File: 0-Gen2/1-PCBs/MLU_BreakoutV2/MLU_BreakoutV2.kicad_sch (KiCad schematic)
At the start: 17 parts, among them J13 SBH11-PBPC-D10-ST-BK, J7 SBH11-PBPC-D10-ST-BK, U6 Teensy4.1

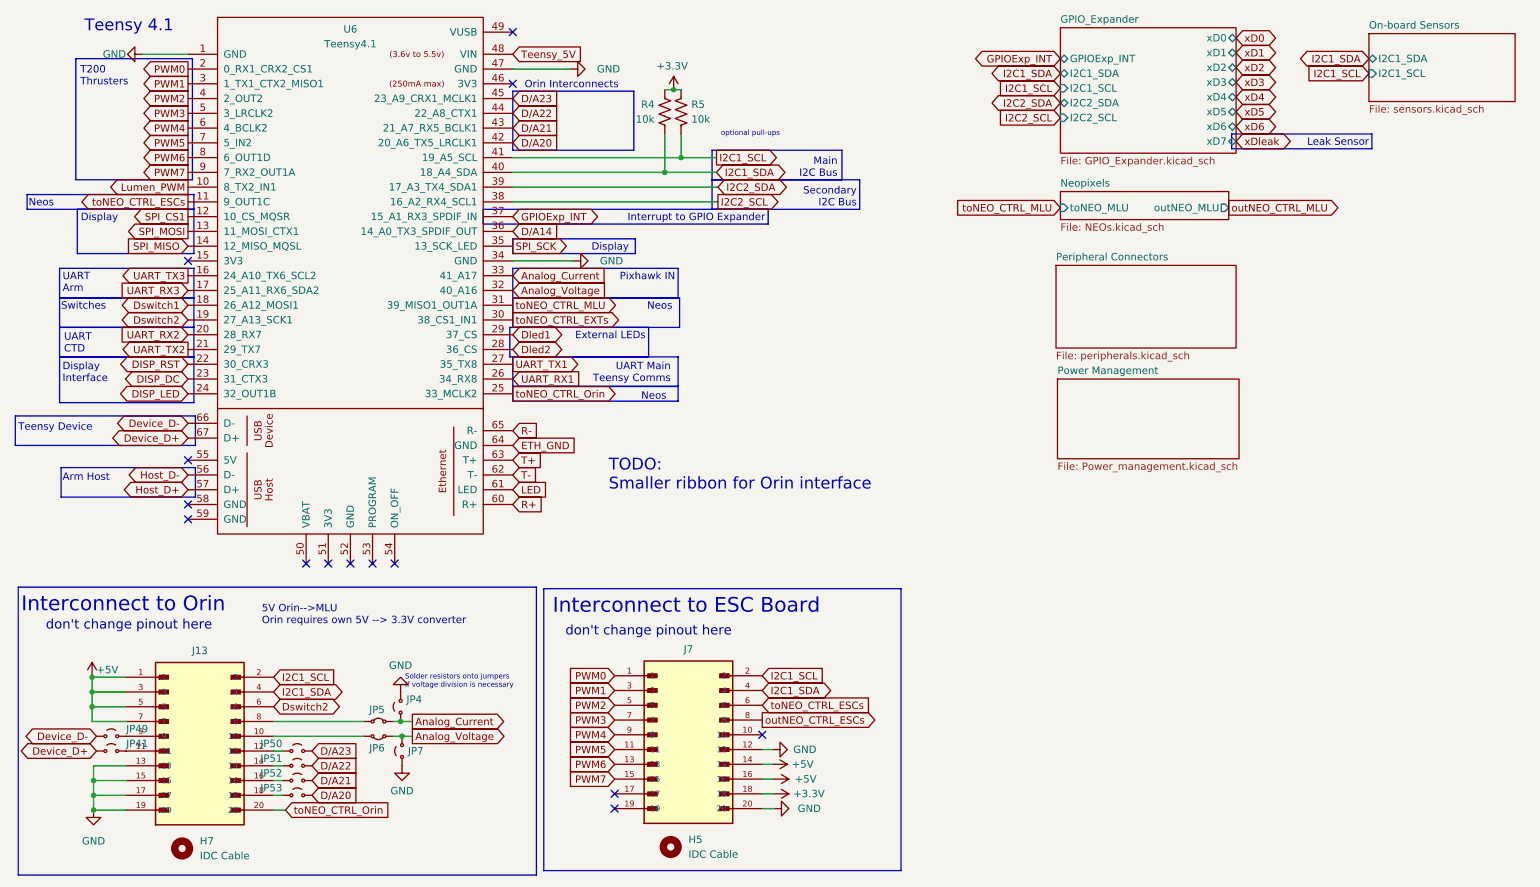
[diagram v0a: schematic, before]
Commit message: before restructure
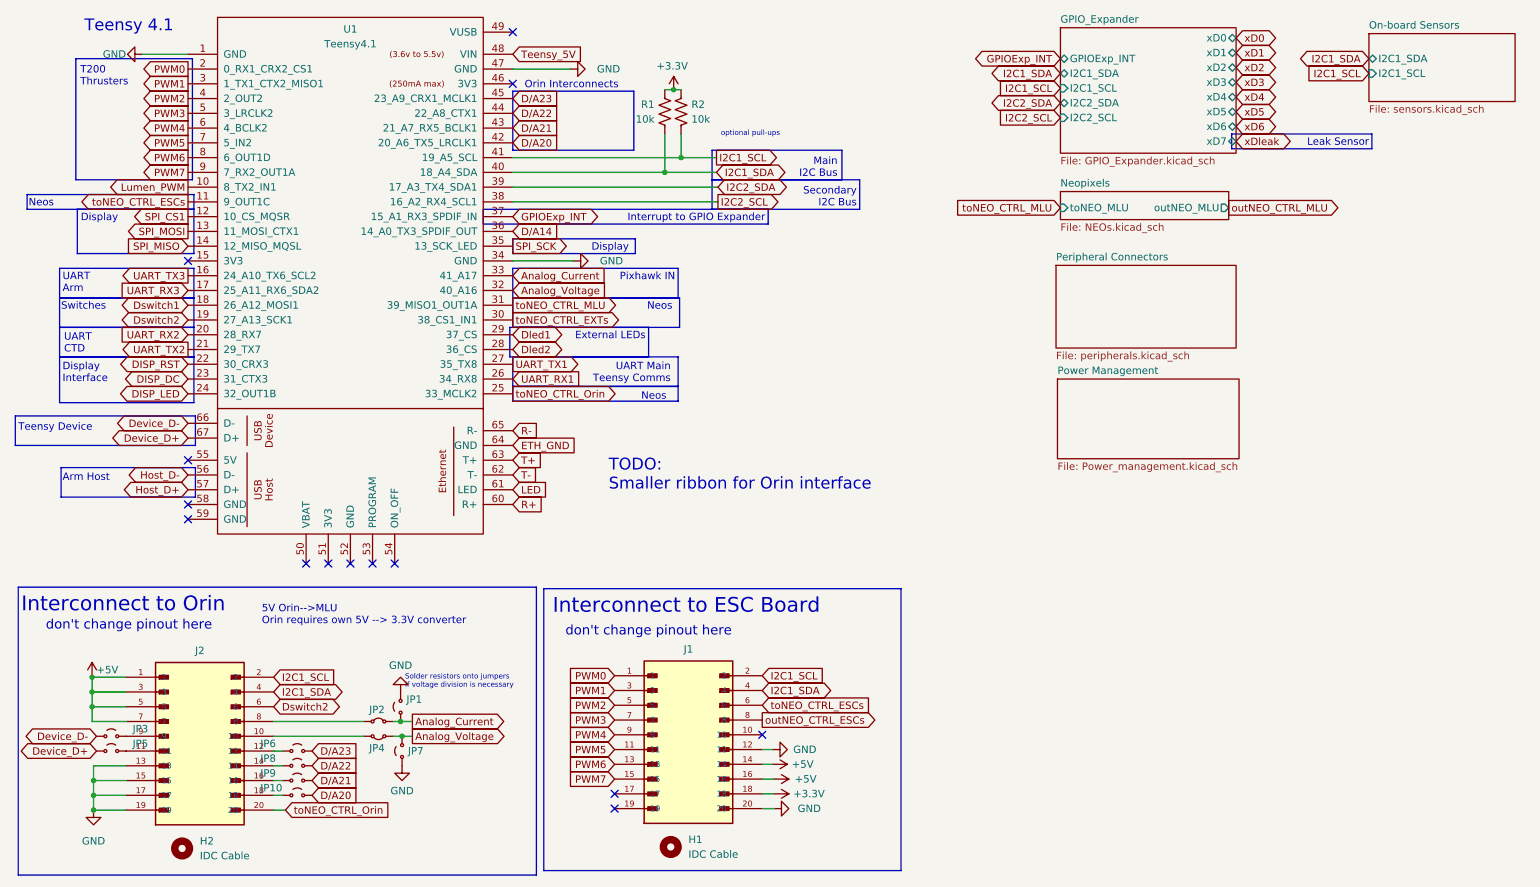
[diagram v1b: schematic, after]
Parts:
- renumbered H5 to H1, H7 to H2, J7 to J1, J13 to J2, JP4 to JP1, JP53 to JP10, JP5 to JP2, JP49 to JP3, JP6 to JP4, JP41 to JP5, JP50 to JP6, JP51 to JP8, JP52 to JP9, R4 to R1, R5 to R2, U6 to U1
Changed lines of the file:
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@@
 		(dnp no)
 		(fields_autoplaced yes)
-		(property "Reference" "#PWR039"
+		(property "Reference" "#PWR04"
 			(at 116.84 56.388 0)
 			(effects
@@
 			(project "MLU_BreakoutV2"
 				(path "/55121ba7-5d22-4fe3-93aa-7f76d75b410c"
-					(reference "#PWR039")
+					(reference "#PWR04")
 					(unit 1)
 				)
@@
 		(on_board yes)
 		(dnp no)
-		(property "Reference" "U6"
+		(property "Reference" "U1"
 			(at 72.136 16.51 0)
 			(effects
@@
 			(project "MLU_BreakoutV2"
 				(path "/55121ba7-5d22-4fe3-93aa-7f76d75b410c"
-					(reference "U6")
+					(reference "U1")
 					(unit 1)
 				)
@@
 		(on_board yes)
 		(dnp no)
-		(property "Reference" "#PWR027"
+		(property "Reference" "#PWR03"
 			(at 127.762 30.988 0)
 			(effects
@@
 			(project "MLU_BreakoutV2"
 				(path "/55121ba7-5d22-4fe3-93aa-7f76d75b410c"
-					(reference "#PWR027")
+					(reference "#PWR03")
 					(unit 1)
 				)
@@
 		(on_board yes)
 		(dnp no)
-		(property "Reference" "R4"
+		(property "Reference" "R1"
 			(at 124.46 29.4639 0)
 			(effects
@@
 			(project "MLU_BreakoutV2"
 				(path "/55121ba7-5d22-4fe3-93aa-7f76d75b410c"
-					(reference "R4")
+					(reference "R1")
 					(unit 1)
 				)
@@
 		(dnp no)
 		(fields_autoplaced yes)
-		(property "Reference" "H7"
+		(property "Reference" "H2"
 			(at 46.228 156.2099 0)
 			(effects
@@
 			(project "MLU_BreakoutV2"
 				(path "/55121ba7-5d22-4fe3-93aa-7f76d75b410c"
-					(reference "H7")
+					(reference "H2")
 					(unit 1)
 				)
@@
 		(dnp no)
 		(fields_autoplaced yes)
-		(property "Reference" "#PWR063"
+		(property "Reference" "#PWR09"
 			(at 81.026 149.606 0)
 			(effects
@@
 			(project ""
 				(path "/55121ba7-5d22-4fe3-93aa-7f76d75b410c"
-					(reference "#PWR063")
+					(reference "#PWR09")
 					(unit 1)
 				)
@@
 		(dnp no)
 		(fields_autoplaced yes)
-		(property "Reference" "#PWR061"
+		(property "Reference" "#PWR06"
 			(at 80.772 124.206 0)
 			(effects
@@
 			(project ""
 				(path "/55121ba7-5d22-4fe3-93aa-7f76d75b410c"
-					(reference "#PWR061")
+					(reference "#PWR06")
 					(unit 1)
 				)
@@
 		(dnp no)
 		(fields_autoplaced yes)
-		(property "Reference" "#PWR030"
+		(property "Reference" "#PWR010"
 			(at 141.224 145.542 0)
 			(effects
@@
 			(project "MLU_BreakoutV2"
 				(path "/55121ba7-5d22-4fe3-93aa-7f76d75b410c"
-					(reference "#PWR030")
+					(reference "#PWR010")
 					(unit 1)
 				)
@@
 		(on_board yes)
 		(dnp no)
-		(property "Reference" "JP5"
+		(property "Reference" "JP2"
 			(at 76.708 133.604 0)
 			(effects
@@
 			(project ""
 				(path "/55121ba7-5d22-4fe3-93aa-7f76d75b410c"
-					(reference "JP5")
+					(reference "JP2")
 					(unit 1)
 				)
@@
 		(on_board yes)
 		(dnp no)
-		(property "Reference" "#PWR060"
+		(property "Reference" "#PWR05"
 			(at 27.686 131.826 0)
 			(effects
@@
 			(project "MLU_BreakoutV2"
 				(path "/55121ba7-5d22-4fe3-93aa-7f76d75b410c"
-					(reference "#PWR060")
+					(reference "#PWR05")
 					(unit 1)
 				)
@@
 		(on_board yes)
 		(dnp no)
-		(property "Reference" "JP50"
+		(property "Reference" "JP6"
 			(at 56.642 139.446 0)
 			(effects
@@
 			(project "MLU_BreakoutV2"
 				(path "/55121ba7-5d22-4fe3-93aa-7f76d75b410c"
-					(reference "JP50")
+					(reference "JP6")
 					(unit 1)
 				)
@@
 		(dnp no)
 		(fields_autoplaced yes)
-		(property "Reference" "#PWR028"
+		(property "Reference" "#PWR07"
 			(at 151.13 140.462 0)
 			(effects
@@
 			(project "MLU_BreakoutV2"
 				(path "/55121ba7-5d22-4fe3-93aa-7f76d75b410c"
-					(reference "#PWR028")
+					(reference "#PWR07")
 					(unit 1)
 				)
@@
 		(on_board yes)
 		(dnp no)
-		(property "Reference" "JP4"
+		(property "Reference" "JP1"
 			(at 81.788 131.826 90)
 			(effects
@@
 			(project ""
 				(path "/55121ba7-5d22-4fe3-93aa-7f76d75b410c"
-					(reference "JP4")
+					(reference "JP1")
 					(unit 1)
 				)
@@
 		(on_board yes)
 		(dnp no)
-		(property "Reference" "R5"
+		(property "Reference" "R2"
 			(at 130.81 29.4639 0)
 			(effects
@@
 			(project "MLU_BreakoutV2"
 				(path "/55121ba7-5d22-4fe3-93aa-7f76d75b410c"
-					(reference "R5")
+					(reference "R2")
 					(unit 1)
 				)
@@
 		(on_board yes)
 		(dnp no)
-		(property "Reference" "J13"
+		(property "Reference" "J2"
 			(at 46.228 123.444 0)
 			(effects
@@
 			(project "MLU_BreakoutV2"
 				(path "/55121ba7-5d22-4fe3-93aa-7f76d75b410c"
-					(reference "J13")
+					(reference "J2")
 					(unit 1)
 				)
@@
 		(on_board yes)
 		(dnp no)
-		(property "Reference" "#PWR026"
+		(property "Reference" "#PWR02"
 			(at 116.332 23.368 0)
 			(effects
@@
 			(project "MLU_BreakoutV2"
 				(path "/55121ba7-5d22-4fe3-93aa-7f76d75b410c"
-					(reference "#PWR026")
+					(reference "#PWR02")
 					(unit 1)
 				)
@@
 		(on_board yes)
 		(dnp no)
-		(property "Reference" "JP53"
+		(property "Reference" "JP10"
 			(at 56.642 147.066 0)
 			(effects
@@
 			(project "MLU_BreakoutV2"
 				(path "/55121ba7-5d22-4fe3-93aa-7f76d75b410c"
-					(reference "JP53")
+					(reference "JP10")
 					(unit 1)
 				)
@@
 		(on_board yes)
 		(dnp no)
-		(property "Reference" "J7"
+		(property "Reference" "J1"
 			(at 130.302 123.19 0)
 			(effects
@@
 			(project "MLU_BreakoutV2"
 				(path "/55121ba7-5d22-4fe3-93aa-7f76d75b410c"
-					(reference "J7")
+					(reference "J1")
 					(unit 1)
 				)
@@
 		(on_board yes)
 		(dnp no)
-		(property "Reference" "JP6"
+		(property "Reference" "JP4"
 			(at 76.708 140.208 0)
 			(effects
@@
 			(project "MLU_BreakoutV2"
 				(path "/55121ba7-5d22-4fe3-93aa-7f76d75b410c"
-					(reference "JP6")
+					(reference "JP4")
 					(unit 1)
 				)
@@
 		(on_board yes)
 		(dnp no)
-		(property "Reference" "JP51"
+		(property "Reference" "JP8"
 			(at 56.642 141.986 0)
 			(effects
@@
 			(project "MLU_BreakoutV2"
 				(path "/55121ba7-5d22-4fe3-93aa-7f76d75b410c"
-					(reference "JP51")
+					(reference "JP8")
 					(unit 1)
 				)
@@
 		(on_board yes)
 		(dnp no)
-		(property "Reference" "JP49"
+		(property "Reference" "JP3"
 			(at 37.338 136.906 0)
 			(effects
@@
 			(project "MLU_BreakoutV2"
 				(path "/55121ba7-5d22-4fe3-93aa-7f76d75b410c"
-					(reference "JP49")
+					(reference "JP3")
 					(unit 1)
 				)
@@
 		(dnp no)
 		(fields_autoplaced yes)
-		(property "Reference" "#PWR034"
+		(property "Reference" "#PWR012"
 			(at 151.384 150.622 0)
 			(effects
@@
 			(project "MLU_BreakoutV2"
 				(path "/55121ba7-5d22-4fe3-93aa-7f76d75b410c"
-					(reference "#PWR034")
+					(reference "#PWR012")
 					(unit 1)
 				)
@@
 		(dnp no)
 		(fields_autoplaced yes)
-		(property "Reference" "#PWR025"
+		(property "Reference" "#PWR01"
 			(at 29.972 20.828 0)
 			(effects
@@
 			(project ""
 				(path "/55121ba7-5d22-4fe3-93aa-7f76d75b410c"
-					(reference "#PWR025")
+					(reference "#PWR01")
 					(unit 1)
 				)
@@
 		(on_board yes)
 		(dnp no)
-		(property "Reference" "JP41"
+		(property "Reference" "JP5"
 			(at 37.338 139.446 0)
 			(effects
@@
 			(project "MLU_BreakoutV2"
 				(path "/55121ba7-5d22-4fe3-93aa-7f76d75b410c"
-					(reference "JP41")
+					(reference "JP5")
 					(unit 1)
 				)
@@
 		(dnp no)
 		(fields_autoplaced yes)
-		(property "Reference" "#PWR064"
+		(property "Reference" "#PWR013"
 			(at 27.94 157.226 0)
 			(effects
@@
 			(project "MLU_BreakoutV2"
 				(path "/55121ba7-5d22-4fe3-93aa-7f76d75b410c"
-					(reference "#PWR064")
+					(reference "#PWR013")
 					(unit 1)
 				)
@@
 		(dnp no)
 		(fields_autoplaced yes)
-		(property "Reference" "#PWR032"
+		(property "Reference" "#PWR011"
 			(at 141.224 148.082 0)
 			(effects
@@
 			(project "MLU_BreakoutV2"
 				(path "/55121ba7-5d22-4fe3-93aa-7f76d75b410c"
-					(reference "#PWR032")
+					(reference "#PWR011")
 					(unit 1)
 				)
@@
 		(dnp no)
 		(fields_autoplaced yes)
-		(property "Reference" "H5"
+		(property "Reference" "H1"
 			(at 130.302 155.9559 0)
 			(effects
@@
 			(project "MLU_BreakoutV2"
 				(path "/55121ba7-5d22-4fe3-93aa-7f76d75b410c"
-					(reference "H5")
+					(reference "H1")
 					(unit 1)
 				)
@@
 		(dnp no)
 		(fields_autoplaced yes)
-		(property "Reference" "#PWR029"
+		(property "Reference" "#PWR08"
 			(at 140.97 143.002 0)
 			(effects
@@
 			(project "MLU_BreakoutV2"
 				(path "/55121ba7-5d22-4fe3-93aa-7f76d75b410c"
-					(reference "#PWR029")
+					(reference "#PWR08")
 					(unit 1)
 				)
@@
 		(on_board yes)
 		(dnp no)
-		(property "Reference" "JP52"
+		(property "Reference" "JP9"
 			(at 56.642 144.526 0)
 			(effects
@@
 			(project "MLU_BreakoutV2"
 				(path "/55121ba7-5d22-4fe3-93aa-7f76d75b410c"
-					(reference "JP52")
+					(reference "JP9")
 					(unit 1)
 				)
